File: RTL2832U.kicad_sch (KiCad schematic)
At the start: 39 parts, among them U3 RTL2832U, U4 M24C02-WMN

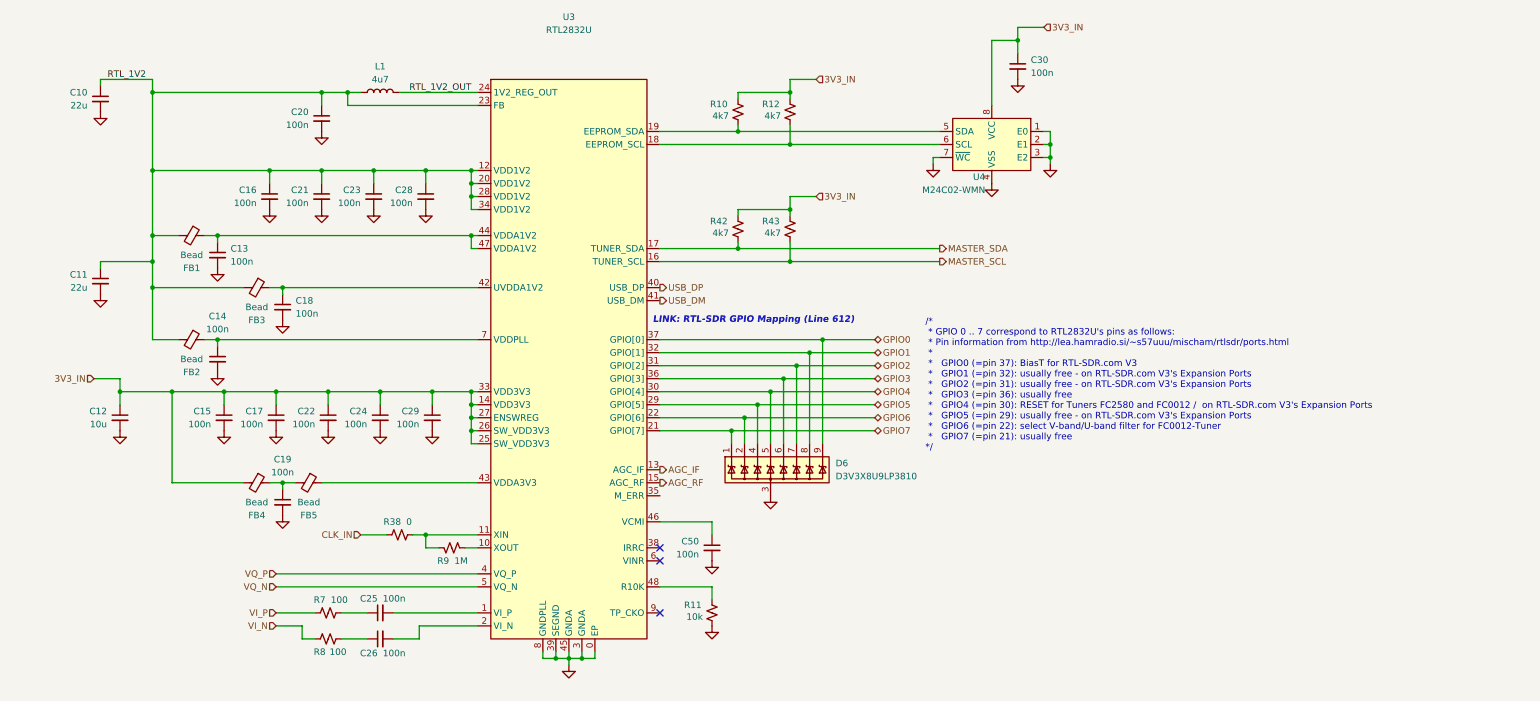
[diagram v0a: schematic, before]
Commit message: Schematic progress
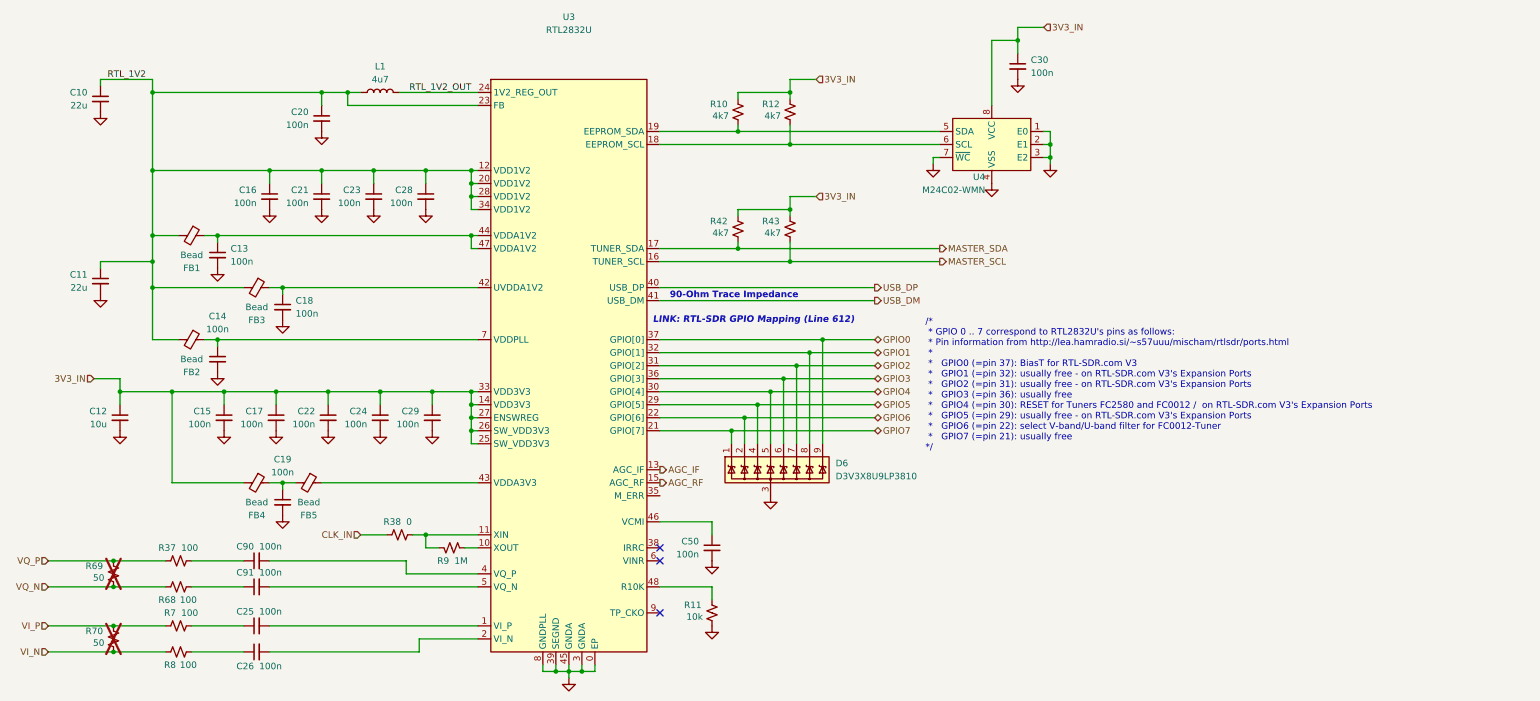
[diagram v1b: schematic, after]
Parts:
- added C90, C91: 100n, libraries:Worthington_C_0402, symbol Device:C_Small
- added R37, R68: 100, libraries:Worthington_R_0402, symbol Device:R_Small_US
- added R69, R70: 50, libraries:Worthington_R_0402, symbol Device:R_Small_US
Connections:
- net VI_N: now also R70.1
- net VI_P: now also R70.2
- net VQ_N: now also R68.2, R69.1; no longer U3.5 (VQ_N)
- net VQ_P: now also R37.1, R69.2; no longer U3.4 (VQ_P)
- new net: C90.1, R37.2
- new net: C90.2, U3.4 (VQ_P)
- new net: C91.2, U3.5 (VQ_N)
- new net: C91.1, R68.1
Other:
- note added: "90-Ohm Trace Impedance"
- moved on the sheet: C25, C26, R7, R8, U3

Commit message: Schematic progress
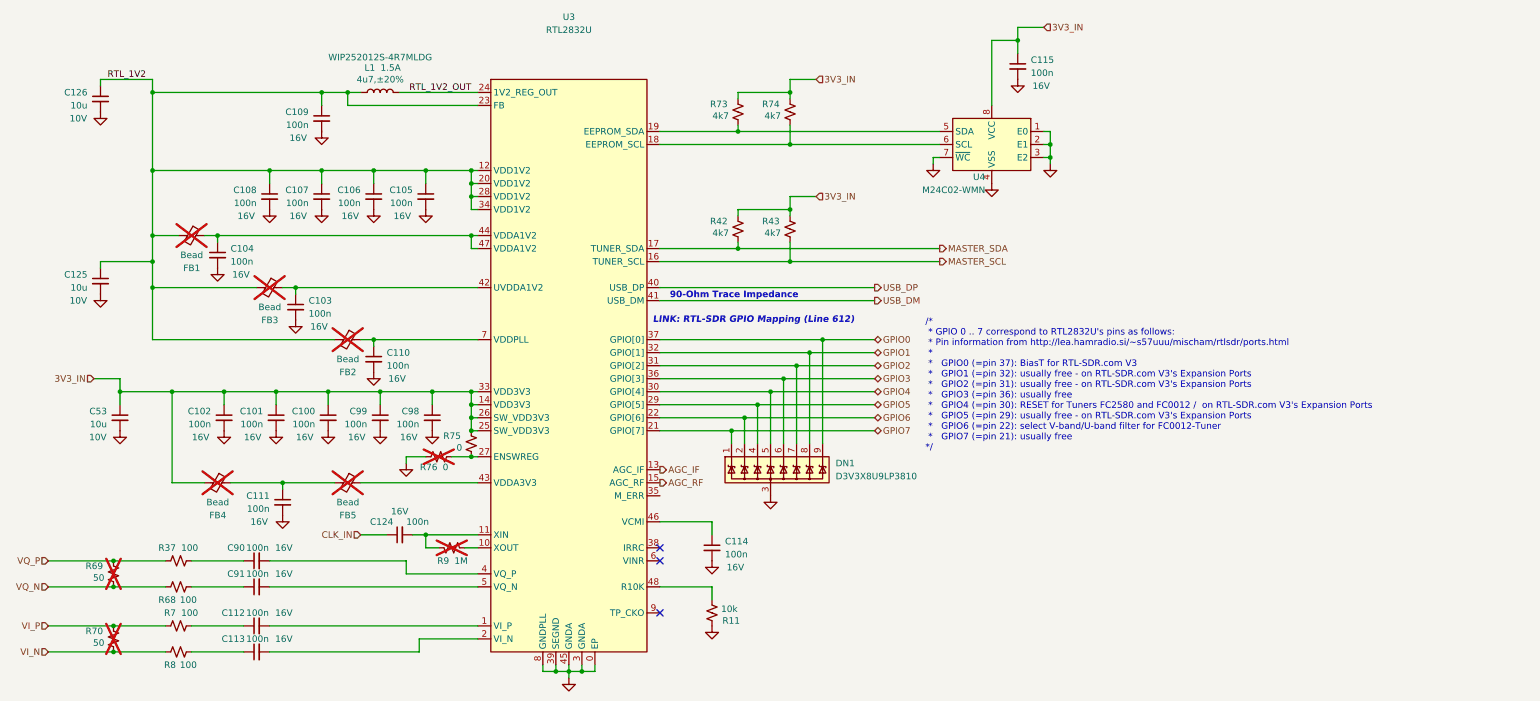
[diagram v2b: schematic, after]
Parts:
- removed C10, C11: 22u, libraries:Worthington_C_0603, symbol Device:C_Small
- removed C12: 10u, libraries:Worthington_C_0603, symbol Device:C_Small
- removed C13, C14, C15, C16, C17, C18, C19, C20, C21, C22, C23, C24, C25, C26, C28, C29, C30, C50: 100n, libraries:Worthington_C_0402, symbol Device:C_Small
- removed R10, R12: 4k7, libraries:Worthington_R_0402, symbol Device:R_Small_US
- removed R38: 0, libraries:Worthington_R_0402, symbol Device:R_Small_US
- added C100, C101, C102, C103, C104, C105, C106, C107, C108, C109, C110, C111, C112, C113, C114, C115, C124, C98, C99: 100n, libraries:Worthington_C_0201, symbol Device:C_Small
- added C125, C126, C53: 10u, libraries:Worthington_C_0402, symbol Device:C_Small
- added R73, R74: 4k7, libraries:Worthington_R_0201, symbol Device:R_Small_US
- added R75, R76: 0, libraries:Worthington_R_0201, symbol Device:R_Small_US
- C90, C91: footprint libraries:Worthington_C_0402 -> libraries:Worthington_C_0201; DigiKey (none) -> 445-15903-1-ND; Manufacturer Part Number (none) -> C0603X6S1C104K030BC; Voltage (none) -> 16V
- FB1, FB2, FB3, FB4, FB5: footprint (none) -> libraries:Worthington_L_0402; now not fitted
- L1: value 4u7 -> 4u7,±20%; footprint Inductor_SMD:L_0805_2012Metric -> Inductor_SMD:L_1008_2520Metric; Current (none) -> 1.5A; DC Resistance (none) -> 180 mOhm; DigiKey (none) -> 3526-WIP252012S-4R7MLDGCT-ND; Manufacturer Part Number (none) -> WIP252012S-4R7MLDG
- R11, R37, R42, R43, R68, R7, R8: footprint libraries:Worthington_R_0402 -> libraries:Worthington_R_0201
- R9: footprint libraries:Worthington_R_0402 -> libraries:Worthington_R_0201; now not fitted
- renumbered D6 to DN1
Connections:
- net 3V3_IN: now also C100.1, C101.1, C102.1, C115.1, C53.1, C98.1, C99.1, R73.2, R74.2, R75.2; no longer U3.27 (ENSWREG)
- net CLK_IN: now also C124.1
- net GND: now also R11.2, C100.2, C101.2, C102.2, C103.2, C104.2, C105.2, C106.2, C107.2, C108.2, C109.2, C110.2, C111.2, C114.2, C115.2, C125.2, C126.2, C53.2, C98.2, C99.2, R76.2; no longer R11.1
- net RTL_1V2: now also C105.1, C106.1, C107.1, C108.1, C109.1, C125.1, C126.1
- net at R7.2: now also C112.1
- net at U3.18 (EEPROM_SCL), U4.6 (SCL): now also R74.1
- net at U3.1 (VI_P): now also C112.2
- net at R9.1, U3.11 (XIN): now also C124.2
- net at U3.48 (R10K): now also R11.1; no longer R11.2
- net at FB4.1, FB5.2: now also C111.1
- net at U3.19 (EEPROM_SDA), U4.5 (SDA): now also R73.1
- net at U3.2 (VI_N): now also C113.2
- net at FB3.1, U3.42 (UVDDA1V2): now also C103.1
- net at FB1.1, U3.44 (VDDA1V2), U3.47 (VDDA1V2): now also C104.1
- net at U3.46 (VCMI): now also C114.1
- net at FB2.1, U3.7 (VDDPLL): now also C110.1
- net at R8.1: now also C113.1
- new net: R75.1, R76.1, U3.27 (ENSWREG)
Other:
- moved on the sheet: R11
